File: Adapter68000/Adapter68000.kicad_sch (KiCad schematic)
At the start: 52 parts, among them P21 Conn_01x20_Male, P22 Service-Tast., Q1 BC327, U1 74HC107, U2 74HC165, U3 74HC4094, U4 74HC4094

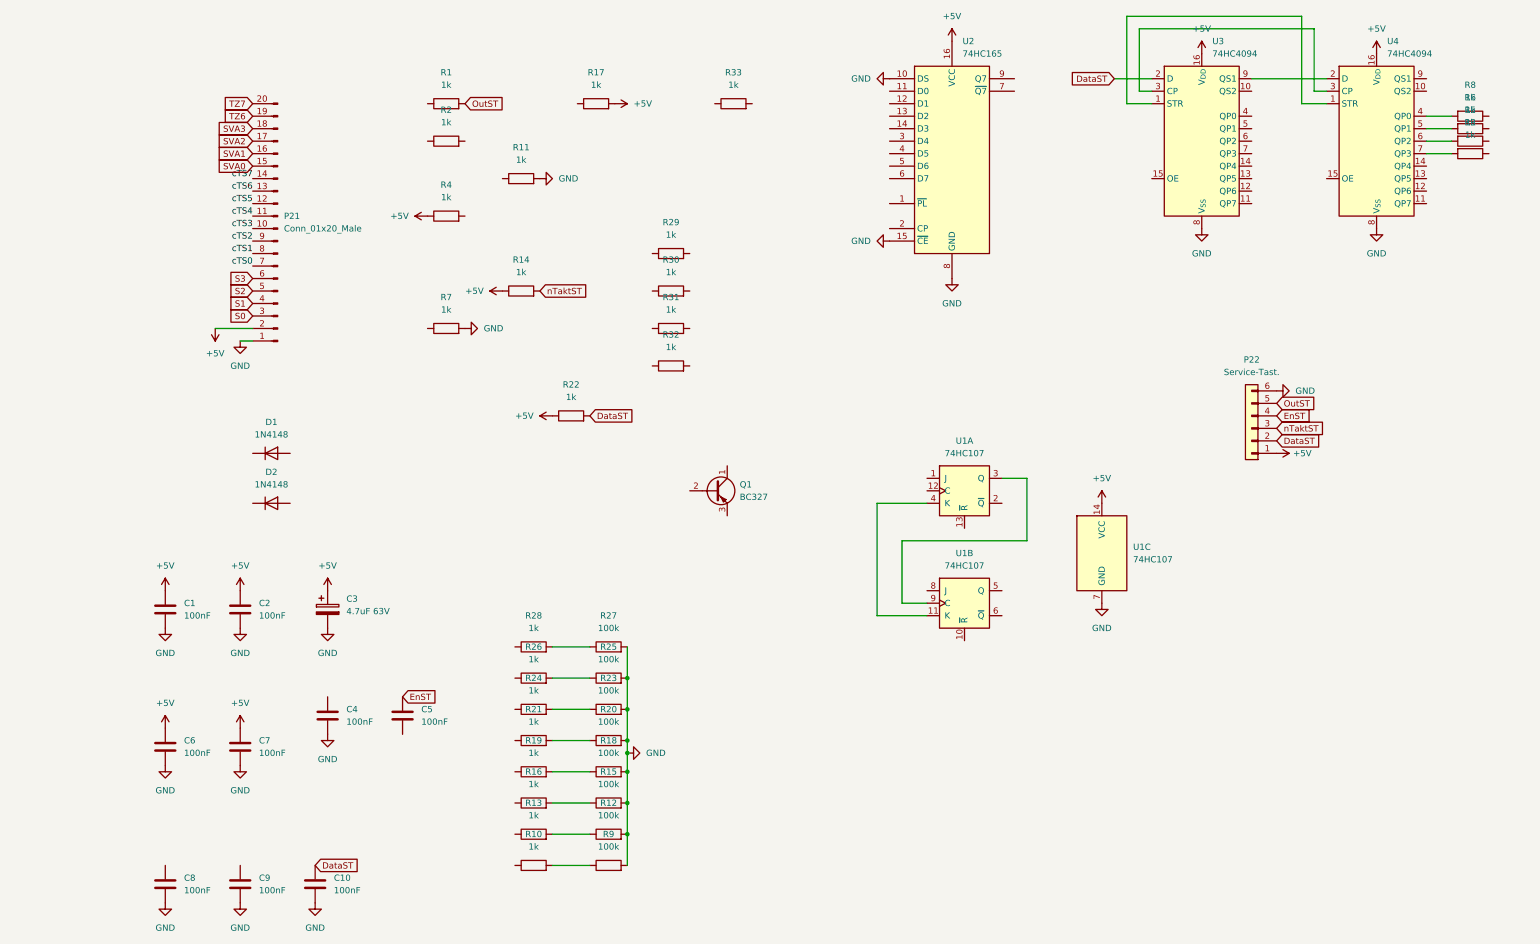
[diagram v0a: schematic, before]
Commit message: diode
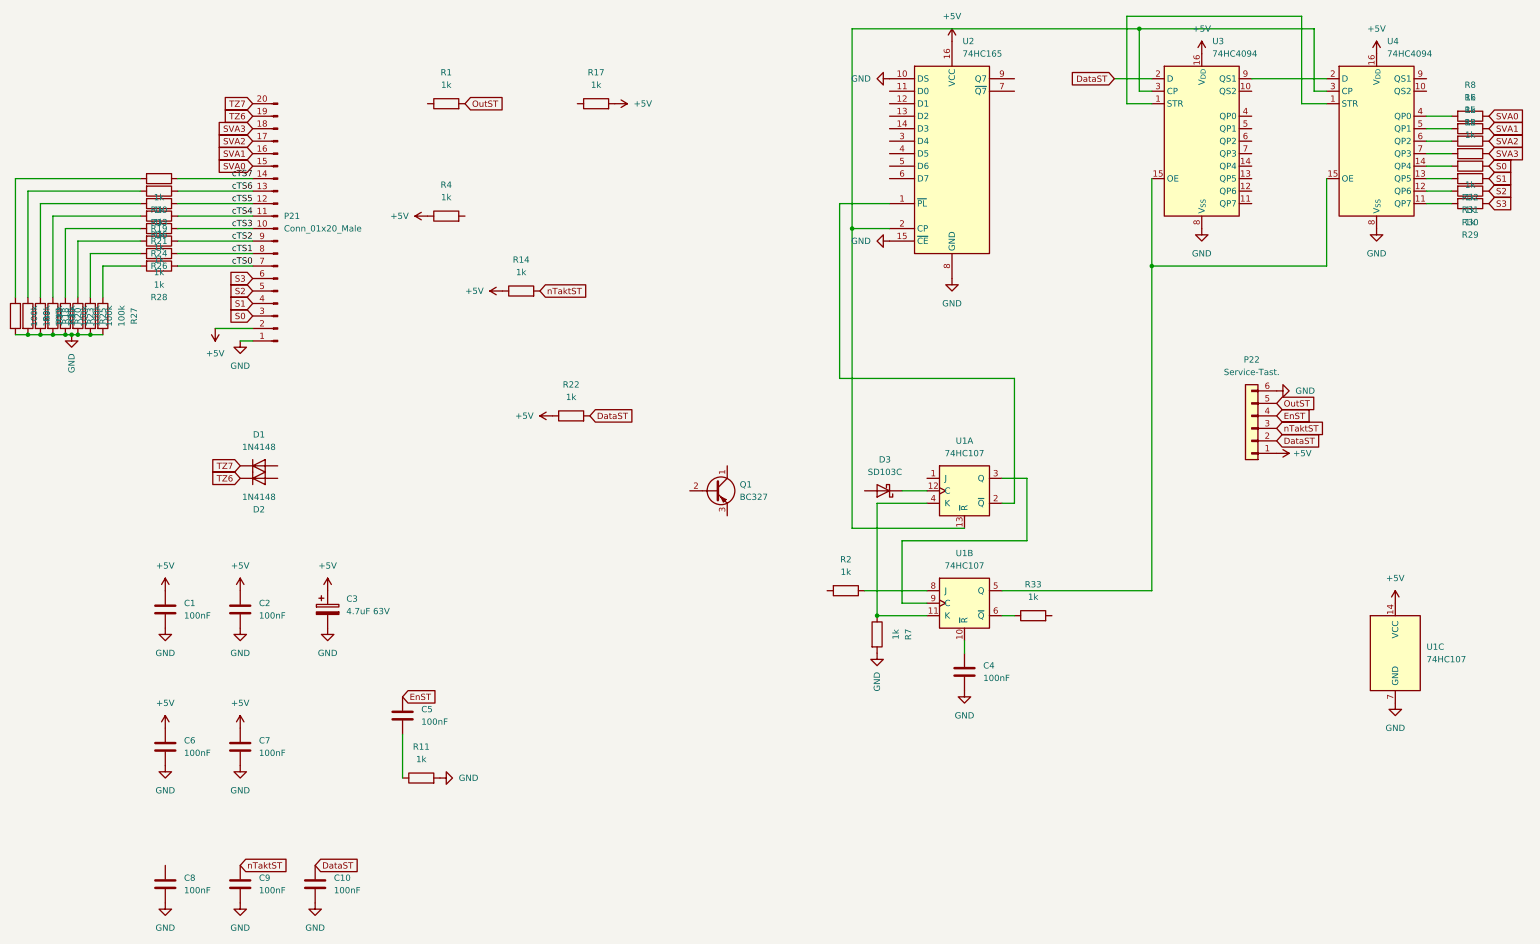
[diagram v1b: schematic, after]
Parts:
- added D3: SD103C, Diode_THT:D_DO-35_SOD27_P7.62mm_Horizontal, symbol Device:D_Schottky
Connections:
- net S0: now also R32.1
- net S1: now also R31.1
- net S2: now also R30.1
- net S3: now also R29.1
- net SVA0: now also R8.1
- net SVA1: now also R6.1
- net SVA2: now also R5.1
- net SVA3: now also R3.1
- net TZ6: now also D2.1 (K)
- net TZ7: now also D1.1 (K)
- net cTS0: now also R28.1
- net cTS1: now also R26.1
- net cTS2: now also R24.1
- net cTS3: now also R21.1
- net cTS4: now also R19.1
- net cTS5: now also R16.1
- net cTS6: now also R13.1
- net cTS7: now also R10.1
- net nTaktST: now also C9.2
- net at C4.2: now also U1.10 (~{R})
- net at U2.1 (~{PL}): now also U1.2 (~{Q})
- net at U2.2 (CP): now also U1.13 (~{R}), U3.3 (CP), U4.3 (CP)
- net at R31.2: now also U4.13 (QP5)
- net at U1.12 (C): now also D3.1 (K)
- net at U1.11 (K), U1.4 (K): now also R7.1
- net at R33.1: now also U1.6 (~{Q})
- net at R32.2: now also U4.14 (QP4)
- net at R11.1: now also C5.1
- net at R30.2: now also U4.12 (QP6)
- net at U1.5 (Q): now also U3.15 (OE), U4.15 (OE)
- net at U1.8 (J): now also R2.1
- net at U4.11 (QP7): now also R29.2
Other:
- moved on the sheet: C4, D1, D2, R10, R11, R12, R13, R15, R16, R18, R19, R2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

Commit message: kompletti
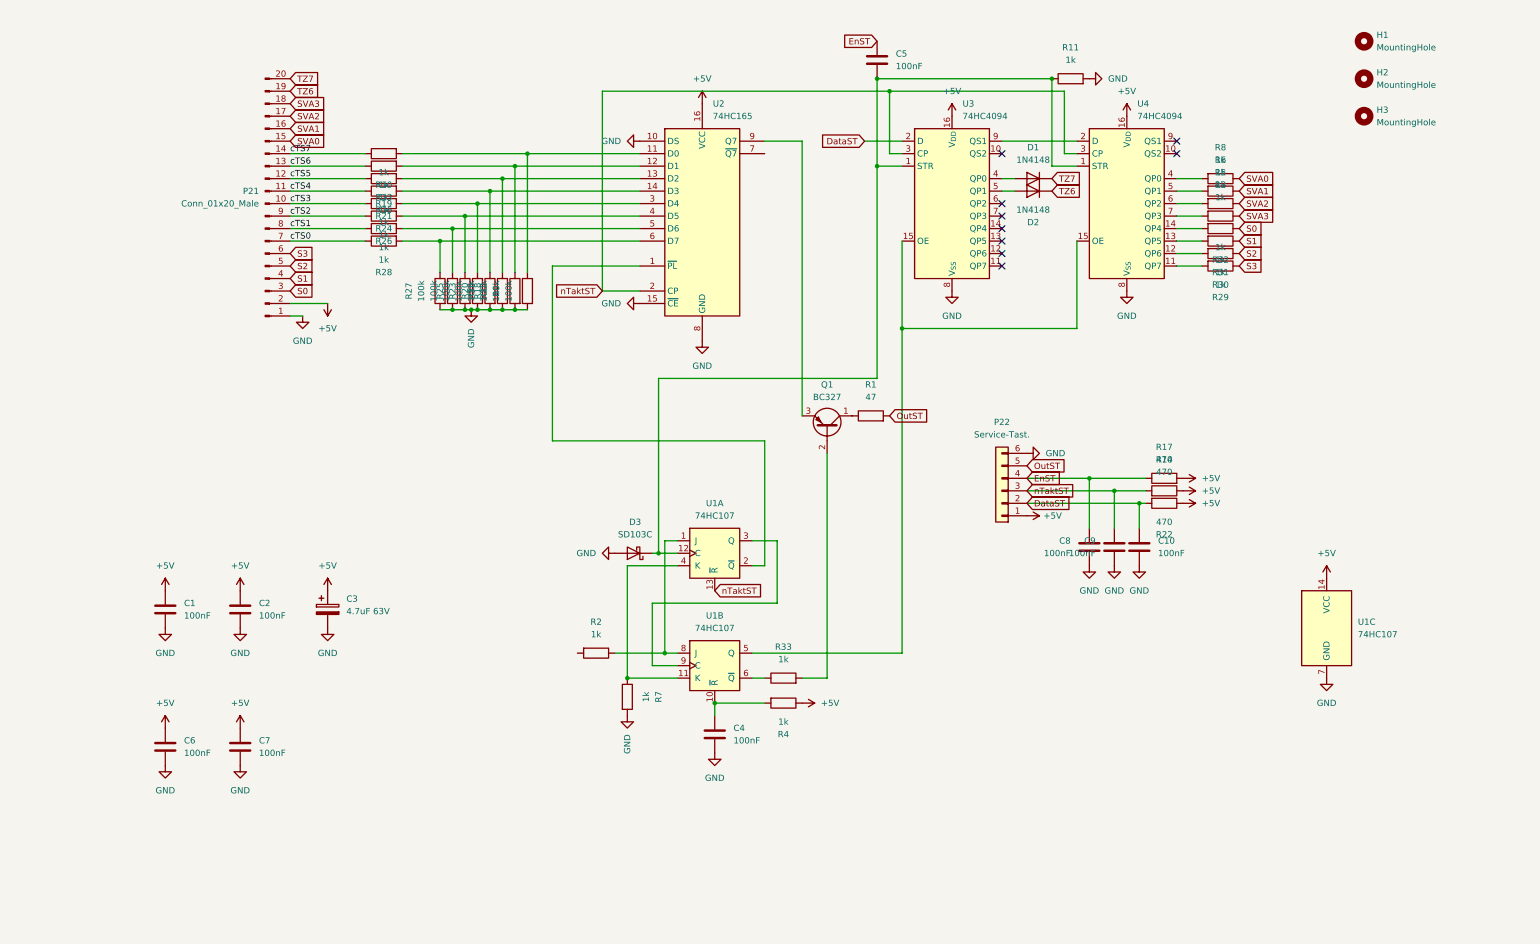
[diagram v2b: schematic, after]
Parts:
- added H1, H2, H3: MountingHole, MountingHole:MountingHole_3.2mm_M3, symbol Mechanical:MountingHole
- R1: value 1k -> 47
- R14, R17, R22: value 1k -> 470
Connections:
- net EnST: now also C8.2, R17.1
- net GND: now also D3.2 (A)
- net nTaktST: now also U1.13 (~{R}), U2.2 (CP), U3.3 (CP), U4.3 (CP)
- net at R10.2, R9.1: now also U2.11 (D0)
- net at R15.1, R16.2: now also U2.13 (D2)
- net at C4.2, U1.10 (~{R}): now also R4.2
- net at U2.12 (D1): now also R12.1, R13.2
- net at U2.14 (D3): now also R18.1, R19.2
- net at U2.3 (D4): now also R20.1, R21.2
- net at U2.4 (D5): now also R23.1, R24.2
- net at U2.5 (D6): now also R25.1, R26.2
- net at U2.6 (D7): now also R27.1, R28.2
- net at U2.9 (Q7): now also Q1.3 (E)
- net at D2.2 (A): now also U3.5 (QP1)
- net at U1.1 (J): now also R2.1, U1.8 (J)
- net at D3.1 (K), U1.12 (C): now also C5.1, R11.1, U3.1 (STR), U4.1 (STR)
- net at R33.2: now also Q1.2 (B)
- net at R1.1: now also Q1.1 (C)
- net at U3.4 (QP0): now also D1.2 (A)
- no-connect marks 0 -> 9
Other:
- moved on the sheet: C10, C4, C5, C8, C9, D1, D2, D3, P21, P22, Q1, R1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
